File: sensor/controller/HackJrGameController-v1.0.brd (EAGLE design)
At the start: 100 x 80 mm, 37 parts, among them K1 BUTTON-4P-3110040P1, K2 BUTTON-4P-3110040P1, K3 BUTTON-4P-3110040P1, K4 BUTTON-4P-3110040P1, SW1 SWITCH-2CH-6P-3010010P1, SW2 SWITCH-2CH-6P-3010010P1

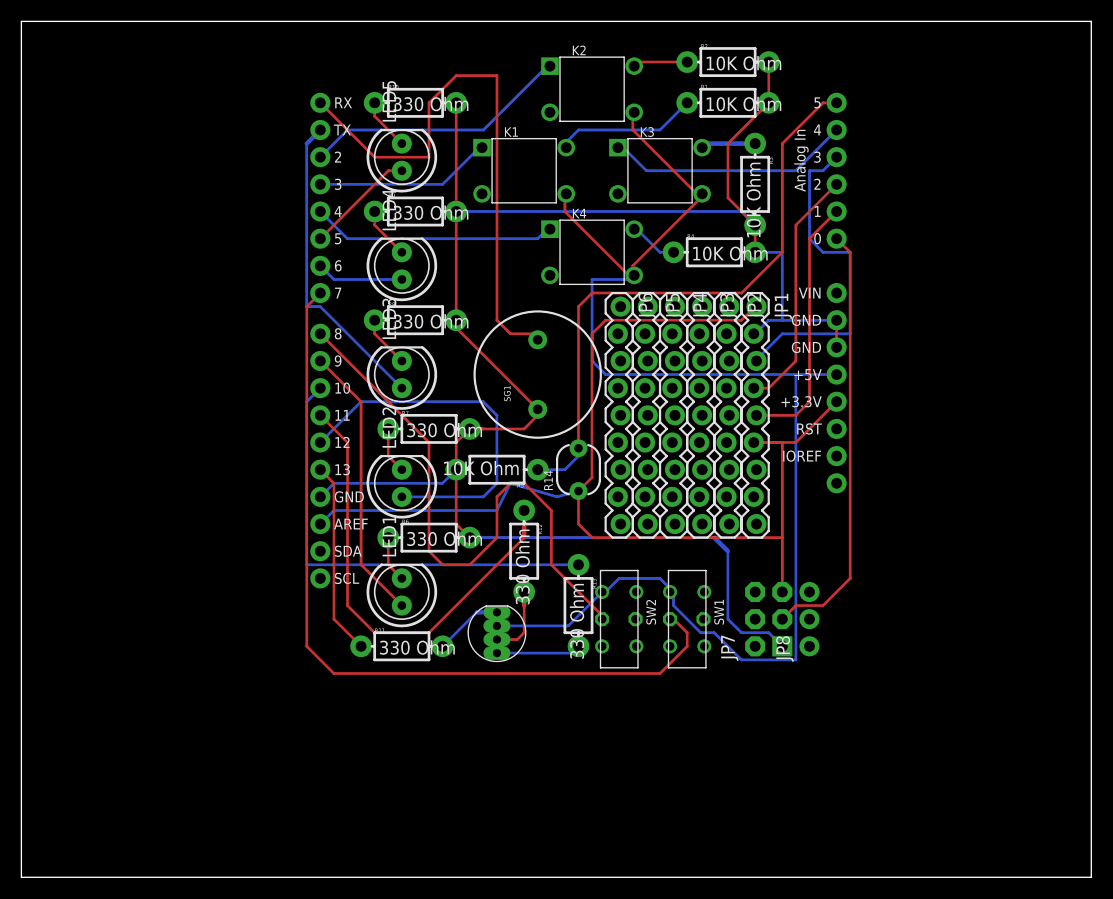
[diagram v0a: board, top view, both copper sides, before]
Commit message: update schematic, layout and new gerber files for manufacturing
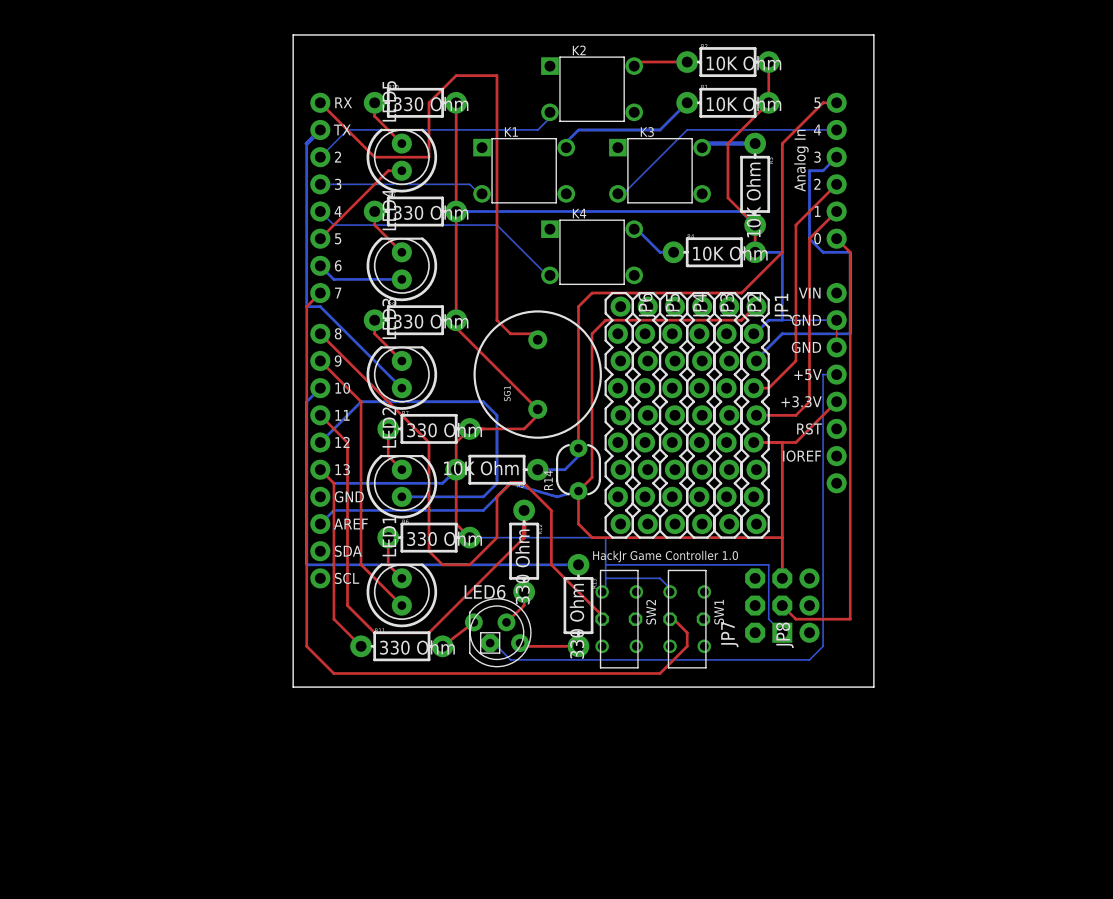
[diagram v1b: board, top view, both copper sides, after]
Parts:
- removed D1: LED-RGB-CA-THRUDIFFUSE, SparkFun-LED:LED-RGB-THRU
- added LED6: RGBLED_CA-5MM, adafruit:LED5MMRGB
- moved FRAME1 124.0 mm to (20.3, 1.27)
- moved JP7 1.27 mm to (69.8, 25.4)
- moved JP8 1.27 mm to (73.7, 22.9)
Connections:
- removed net N$21: K1.1, U$1.D3
- new net N$40: K1.2, U$1.D3
- net N$1: now also LED6.2; no longer D1.2, K1.3, K2.3, K3.3, K4.3, SW1.CH1A, SW2.CH1A
- net N$2: now also SW1.CH1A, SW2.CH1A; no longer U$1.GND@2
- net N$22: now also K2.2; no longer K2.1
- net N$23: now also K3.2; no longer K3.1
- net N$24: now also K4.2; no longer K4.1
- net N$3: now also LED6.1; no longer D1.1
- net N$4: now also LED6.4; no longer D1.4
- net N$5: now also LED6.3; no longer D1.3
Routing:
- net N$1: track 128.3 -> 58.9 mm
- net N$21: track 17.2 -> 0.00 mm
- net N$40: track 0.00 -> 16.2 mm
- net N$2: track 175.0 -> 179.7 mm
- net N$5: track 7.88 -> 3.55 mm
- net N$34: track 40.2 -> 43.0 mm
- net N$3: track 6.40 -> 3.68 mm
- net N$4: track 7.88 -> 5.57 mm
- net N$22: track 25.7 -> 23.6 mm
- net N$19: track 106.7 -> 105.0 mm
- net N$24: track 23.6 -> 24.6 mm
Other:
- board size 100 x 80 mm -> 54.3 x 61 mm
- board text added: "HackJr Game Controller 1.0"
